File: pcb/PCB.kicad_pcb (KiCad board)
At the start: 4 copper layers, 29.2 x 51.1 mm, 35 parts, among them J1 Conn_01x15, J2 USB_C_Receptacle_USB2.0, J3 Conn_01x15, J4 TC2030, J5 Conn_01x04, SW1 SW_Push, SW2 SW_Push, U1 SN65HVD230, U2 AMS1117-3.3, U3 STM32F103C8T6, Y1 8MHz

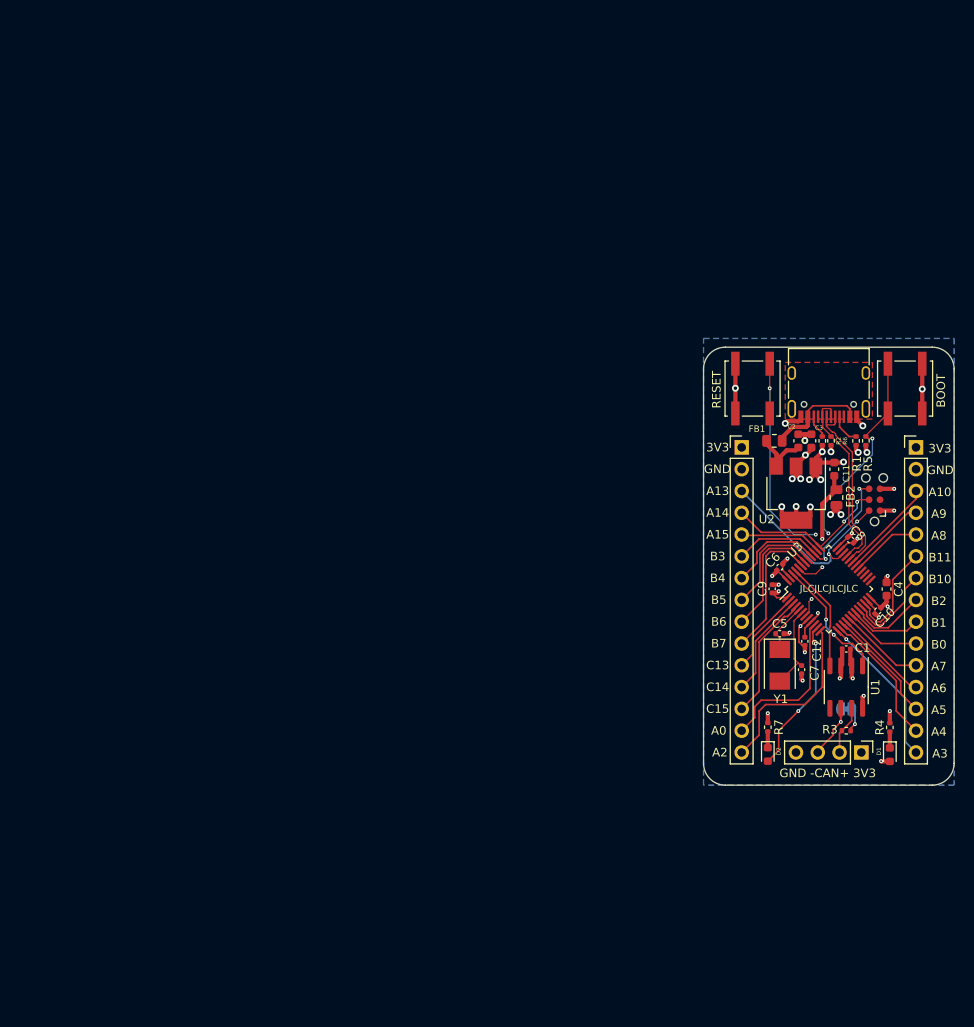
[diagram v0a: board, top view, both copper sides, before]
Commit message: pcb update precharge
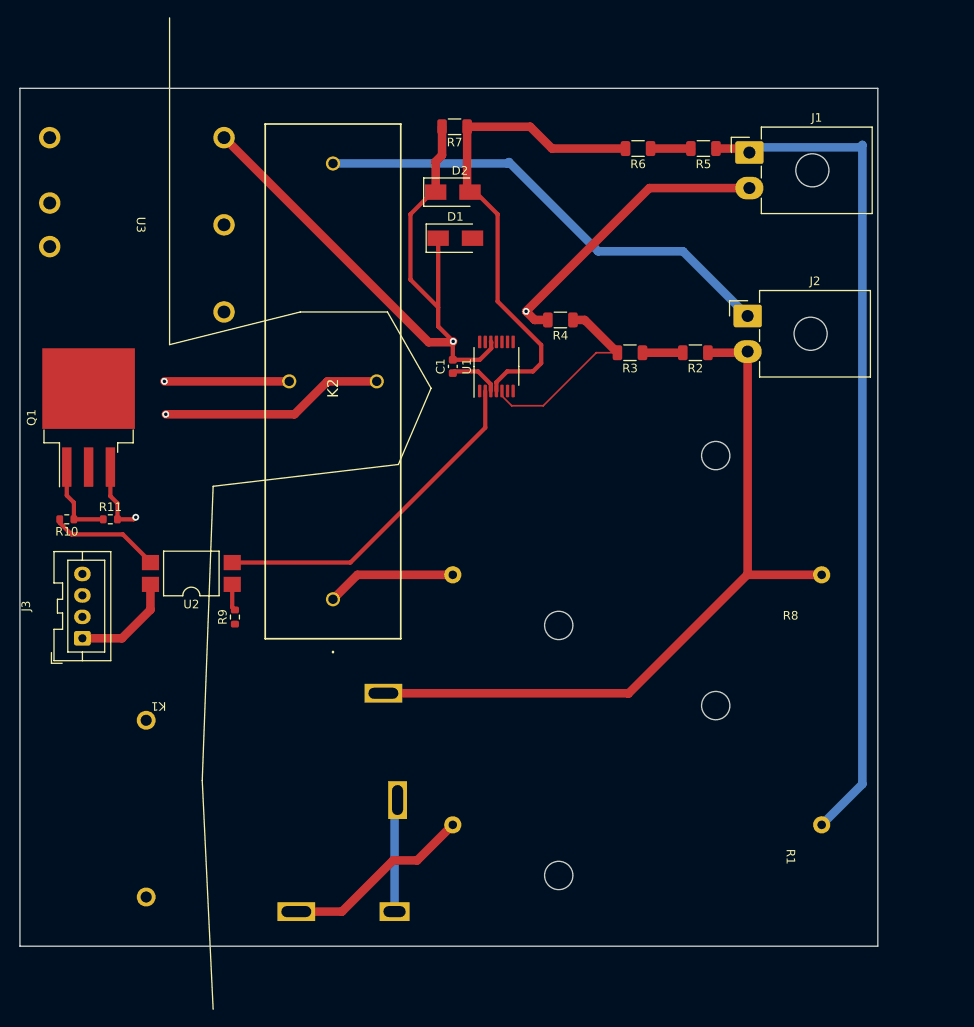
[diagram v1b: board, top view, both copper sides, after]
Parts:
- removed C10, C12, C6, C8, C9: 100n, Capacitor_SMD:C_0402_1005Metric
- removed C11, C2, C3: 1u, Capacitor_SMD:C_0603_1608Metric
- removed C4: 4u7, Capacitor_SMD:C_0603_1608Metric
- removed C5, C7: 30p, Capacitor_SMD:C_0402_1005Metric
- removed FB1, FB2: 100R@100MHz, Resistor_SMD:R_0805_2012Metric
- removed J4: TC2030, Connector:Tag-Connect_TC2030-IDC-NL_2x03_P1.27mm_Vertical
- removed J5: Conn_01x04, Connector_PinHeader_2.54mm:PinHeader_1x04_P2.54mm_Vertical
- removed JP1: SolderJumper_Bridged, Jumper:SolderJumper-2_P1.3mm_Bridged_RoundedPad1.0x1.5mm
- removed SW1, SW2: SW_Push, Button_Switch_SMD:SW_Push_1P1T_NO_CK_KSC7xxJ
- removed Y1: 8MHz, Crystal:Crystal_SMD_5032-2Pin_5.0x3.2mm
- added K1: AZDC6, AZDC6:AZDC6, F.Cu at (64.8, 114.9)
- added K2: dbt71205u21, dbt71205u:DBT71205U, F.Cu at (89.5, 106.6)
- added Q1: IRLZ44N, Package_TO_SOT_SMD:TO-263-3_TabPin2, F.Cu at (61.0, 85.4)
- added R10: 1k, Resistor_SMD:R_0603_1608Metric, F.Cu at (58.5, 97.3)
- added R11: 10K, Resistor_SMD:R_0603_1608Metric, F.Cu at (63.6, 97.3)
- added R8: hsa255k6j, hsa255k6j:hsa255k6j, F.Cu at (150.5, 113.8)
- added R9: 680, Resistor_SMD:R_0603_1608Metric, F.Cu at (78.1, 108.7)
- C1: footprint Capacitor_SMD:C_0402_1005Metric -> Capacitor_SMD:C_0603_1608Metric
- D1: value YELLOW -> SMAJ15CA; footprint LED_SMD:LED_0603_1608Metric -> Diode_SMD:D_SMA
- D2: value BLUE -> SMAJ15CA; footprint LED_SMD:LED_0603_1608Metric -> Diode_SMD:D_SMA
- J1: value Conn_01x15 -> TE 770966-2; footprint Connector_PinHeader_2.54mm:PinHeader_1x15_P2.54mm_Vertical -> Connector_TE-Connectivity:TE_MATE-N-LOK_1-770966-x_1x02_P4.14mm_Horizontal
- J2: value USB_C_Receptacle_USB2.0 -> TE 770966-2; footprint Connector_USB:USB_C_Receptacle_HRO_TYPE-C-31-M-12 -> Connector_TE-Connectivity:TE_MATE-N-LOK_1-770966-x_1x02_P4.14mm_Horizontal
- J3: value Conn_01x15 -> JST B04B-XASK; footprint Connector_PinHeader_2.54mm:PinHeader_1x15_P2.54mm_Vertical -> Connector_JST:JST_XA_B04B-XASK-1_1x04_P2.50mm_Vertical
- R1: value 5k1 -> hsa255k6j; footprint Resistor_SMD:R_0402_1005Metric -> hsa255k6j:hsa255k6j
- R2, R5: value 5k1 -> 5M; footprint Resistor_SMD:R_0402_1005Metric -> Resistor_SMD:R_1206_3216Metric
- R3: value 120R -> 5M; footprint Resistor_SMD:R_0402_1005Metric -> Resistor_SMD:R_1206_3216Metric
- R4: value 1k5 -> 110k; footprint Resistor_SMD:R_0402_1005Metric -> Resistor_SMD:R_1206_3216Metric
- R6: value 1k5 -> 5M; footprint Resistor_SMD:R_0402_1005Metric -> Resistor_SMD:R_1206_3216Metric
- R7: value 1k5 -> 100k; footprint Resistor_SMD:R_0402_1005Metric -> Resistor_SMD:R_1206_3216Metric
- U1: value SN65HVD230 -> LM339; footprint Package_SO:SOIC-8_3.9x4.9mm_P1.27mm -> Package_SO:TSSOP-14_4.4x5mm_P0.65mm
- U2: value AMS1117-3.3 -> LTV-817S; footprint Package_TO_SOT_SMD:SOT-223-3_TabPin2 -> Package_DIP:SMDIP-4_W9.53mm
- U3: value STM32F103C8T6 -> VRB1205YMD-15WR3; footprint Package_QFP:LQFP-48_7x7mm_P0.5mm -> VRB1205YMD-6WR3:VRB1205YMD-15WR3
- moved J3 99.7 mm to (60.3, 111.2), turned to 90 degrees
- moved U3 91.2 mm to (66.7, 63.0), turned to 0 degrees
- moved R7 78.9 mm to (103.7, 51.5), turned to 180 degrees
- moved D1 78.7 mm to (103.8, 64.5), turned to 0 degrees
- moved D2 75.1 mm to (103.5, 59.1), turned to 0 degrees
- moved U2 71.1 mm to (73.0, 103.6), turned to 180 degrees
- moved R4 61.1 mm to (116.0, 74.0), turned to 180 degrees
- moved C1 56.5 mm to (103.5, 79.5), turned to 90 degrees
- moved U1 55.3 mm to (108.6, 79.5), turned to 90 degrees
- moved R1 54.8 mm to (150.5, 142.9), turned to 180 degrees
- moved R3 50.8 mm to (124.1, 77.9), turned to 180 degrees
- moved R6 40.8 mm to (125.1, 54.1), turned to 180 degrees
- moved R5 39.0 mm to (132.7, 54.1), turned to 180 degrees
- moved J1 34.4 mm to (138.1, 54.5)
- moved R2 18.0 mm to (131.8, 77.9), turned to 180 degrees
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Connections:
- C1 pad 1: +3V3 -> +5V
- C1 pad 2: GND -> TS-
- D1 pad 1: Net-(D1-Pad1) -> TS-
- D1 pad 2: +3V3 -> Net-(D1-Pad2)
- D2 pad 1: Net-(D2-Pad1) -> TS-
- D2 pad 2: /LED_STAT -> Net-(D2-Pad2)
- J1 pad 1: +3V3 -> TS+
- J1 pad 2: GND -> TS-
- J3 pad 1: +3V3 -> +12V
- J3 pad 3: PA10 -> Net-(J3-Pad3)
- J3 pad 4: PA9 -> unconnected-(J3-Pad4)
- R1 pad 1: Net-(J2-PadA5) -> TS+
- R1 pad 2: GND -> Net-(K1-Pad1)
- R2 pad 1: GND -> Precharge
- R2 pad 2: Net-(J2-PadB5) -> Net-(R2-Pad2)
- R3 pad 1: /CAN+ -> Net-(R2-Pad2)
- R3 pad 2: Net-(JP1-Pad2) -> Net-(D1-Pad2)
- R4 pad 1: Net-(D1-Pad1) -> Net-(D1-Pad2)
- R4 pad 2: GND -> TS-
- R5 pad 1: /BOOT0 -> TS+
- R5 pad 2: GND -> Net-(R5-Pad2)
- R6 pad 1: +3V3 -> Net-(R5-Pad2)
- R6 pad 2: USB_D+ -> Net-(D2-Pad2)
- R7 pad 1: Net-(D2-Pad1) -> Net-(D2-Pad2)
- R7 pad 2: GND -> TS-
- U1 pad 1: CANTX -> (no net)
- U1 pad 2: GND -> Net-(U1-Pad2)
- U1 pad 3: +3V3 -> +5V
- U1 pad 4: CANRX -> Net-(D2-Pad2)
- U1 pad 5: unconnected-(U1-Pad5) -> Net-(D1-Pad2)
- U1 pad 6: /CAN- -> (no net)
- U1 pad 7: /CAN+ -> (no net)
- U1 pad 8: GND -> (no net)
- U2 pad 1: GND -> Net-(R9-Pad2)
- U2 pad 2: +3V3 -> Net-(U1-Pad2)
- U2 pad 3: VCC -> Net-(R10-Pad2)
- U3 pad 1: +3V3 -> +12V
- U3 pad 2: PC13 -> GND
- U3 pad 3: PC14 -> +12V
- U3 pad 4: PC15 -> +5V
- U3 pad 5: /HSE_OUT -> unconnected-(U3-Pad5)
- U3 pad 6: /HSE_IN -> TS-
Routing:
- net TS-: track 0.00 -> 116.4 mm, vias 0 -> 2
- net TS+: track 0.00 -> 98.9 mm
- net Precharge: track 0.00 -> 87.6 mm
- net Net-(D2-Pad2): track 0.00 -> 58.2 mm
- net Discharge: track 0.00 -> 55.8 mm
- net +3V3: track 44.0 -> 0.00 mm, vias 18 -> 0
- net Net-(U1-Pad2): track 0.00 -> 40.3 mm
- net /NRST: track 35.9 -> 0.00 mm, vias 3 -> 0
- net /BOOT0: track 31.5 -> 0.00 mm, vias 3 -> 0
- net +12V: track 0.00 -> 26.8 mm, vias 0 -> 1
- net SWDIO: track 24.1 -> 0.00 mm, vias 2 -> 0
- net Net-(D1-Pad2): track 0.00 -> 23.8 mm
- net SWO: track 22.9 -> 0.00 mm, vias 2 -> 0
- net Net-(K1-Pad1): track 0.00 -> 22.4 mm
- net USB_D-: track 21.7 -> 0.00 mm
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- added copper zone on In2.Cu, net +12V
- added copper zone on In1.Cu, net TS-
- removed copper zone on In2.Cu, net +3V3
- removed copper zone on B.Cu, net GND
- removed copper zone on F.Cu, net unconnected-(J2-PadS1)
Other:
- board size 29.2 x 51.1 mm -> 100 x 100 mm
- board text removed: "3V3"
- board text removed: "3V3 +CAN- GND"
- board text removed: "A0"
- board text removed: "A10"
- board text removed: "A13"
- board text removed: "A14"
- board text removed: "A15"
- board text removed: "A2"
- board text removed: "A3"
- board text removed: "A4"
- board text removed: "A5"
- board text removed: "A6"
- board text removed: "A7"
- board text removed: "A8"
- board text removed: "A9"
- board text removed: "B0"
- board text removed: "B1"
- board text removed: "B10"
- board text removed: "B11"
- board text removed: "B2"
- board text removed: "B3"
- board text removed: "B4"
- board text removed: "B5"
- board text removed: "B6"
- board text removed: "B7"
- board text removed: "BOOT"
- board text removed: "C13"
- board text removed: "C14"
- board text removed: "C15"
- board text removed: "CAN TERM"
- board text removed: "GND"
- board text removed: "GND -CAN+ 3V3"
- board text removed: "JLCJLCJLCJLC"
- board text removed: "RESET"
- board text removed: "Rev 1"
- board text removed: "STM32F103 CAN/USB-C Jack LeFevre July 2022"
- board text removed: "SWCLK"
- board text removed: "SWDIO"
- board text removed: "SWO"
